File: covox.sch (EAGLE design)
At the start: 26 parts, among them CN1 POWERJACK, IC1 74HCT373N, IC2 74HC164N

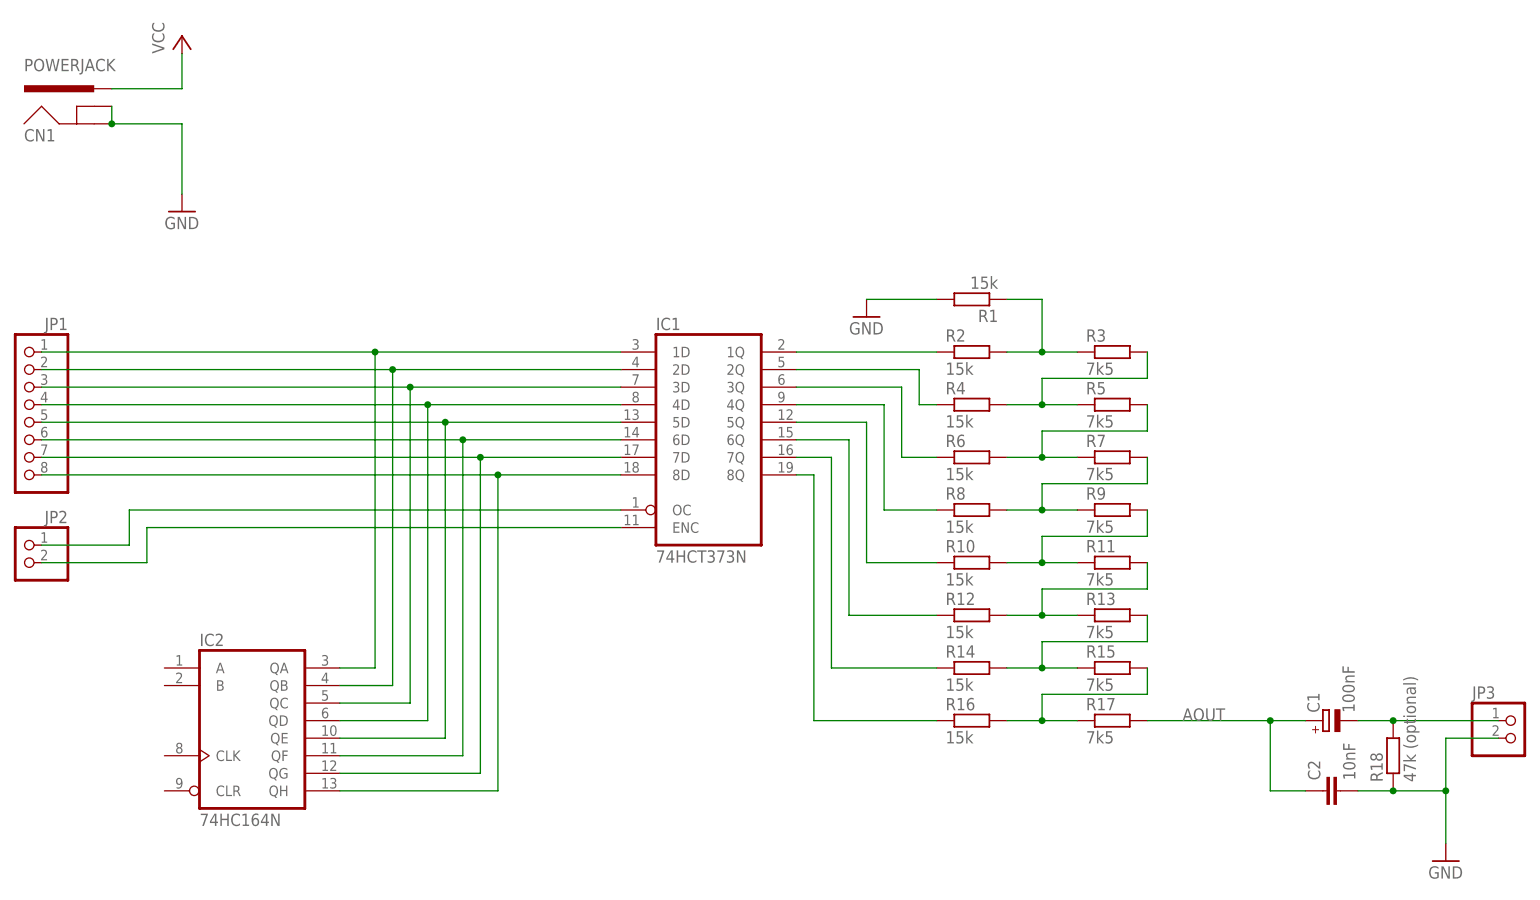
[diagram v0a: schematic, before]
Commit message: Updates...
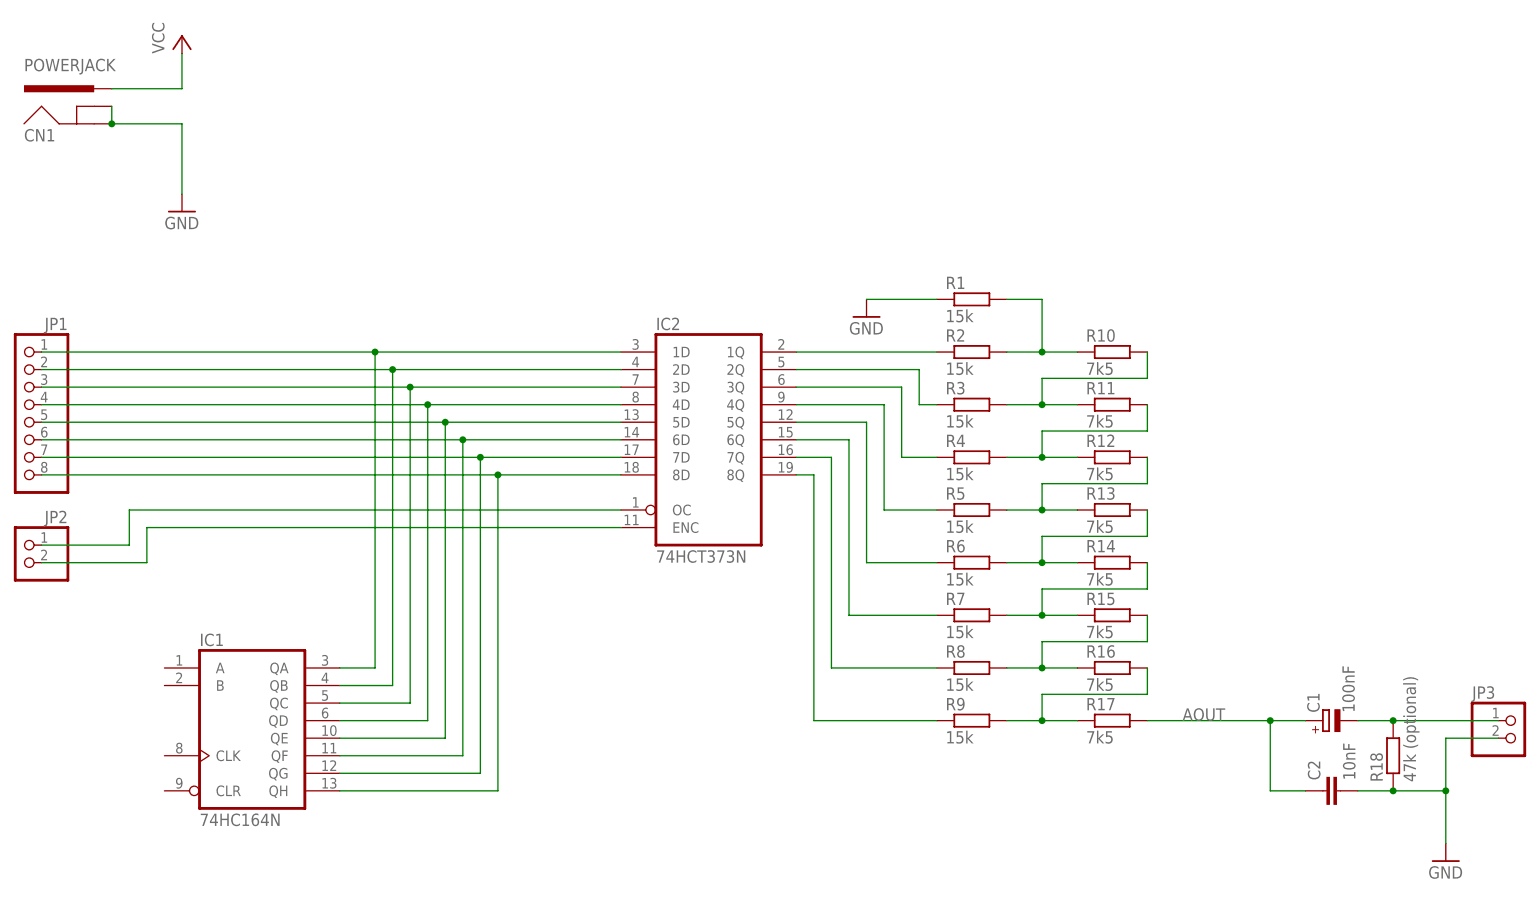
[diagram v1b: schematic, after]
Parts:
- IC1: value 74HCT373N -> 74HC164N; device 74xx-eu:74HCT373N -> 74xx-eu:74HC164N
- IC2: value 74HC164N -> 74HCT373N; device 74xx-eu:74HC164N -> 74xx-eu:74HCT373N
- R10, R12, R14, R16: value 15k -> 7k5
- R3, R5, R7, R9: value 7k5 -> 15k
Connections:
- net GND: now also R1.1; no longer R1.2
- net N$1: now also R1.2, R10.1; no longer R1.1, R3.1
- net N$10: now also IC2A.3Q, R4.1; no longer IC1A.3Q, R6.1
- net N$11: now also IC2A.4Q, R5.1; no longer IC1A.4Q, R8.1
- net N$12: now also IC2A.5Q, R6.1; no longer IC1A.5Q, R10.1
- net N$13: now also IC2A.6Q, R7.1; no longer IC1A.6Q, R12.1
- net N$14: now also IC2A.7Q, R8.1; no longer IC1A.7Q, R14.1
- net N$15: now also IC2A.8Q, R9.1; no longer IC1A.8Q, R16.1
- net N$17: now also R9.2; no longer R15.2
- net N$18: now also IC1A.QA, IC2A.1D; no longer IC1A.1D, IC2A.QA
- net N$19: now also IC1A.QB, IC2A.2D; no longer IC1A.2D, IC2A.QB
- net N$2: now also R10.2, R11.1; no longer R4.2, R5.1
- net N$20: now also IC1A.QC, IC2A.3D; no longer IC1A.3D, IC2A.QC
- net N$21: now also IC1A.QD, IC2A.4D; no longer IC1A.4D, IC2A.QD
- net N$22: now also IC1A.QE, IC2A.5D; no longer IC1A.5D, IC2A.QE
- net N$23: now also IC1A.QF, IC2A.6D; no longer IC1A.6D, IC2A.QF
- net N$24: now also IC1A.QG, IC2A.7D; no longer IC1A.7D, IC2A.QG
- net N$25: now also IC1A.QH, IC2A.8D; no longer IC1A.8D, IC2A.QH
- net N$26: now also IC2A.OC; no longer IC1A.OC
- net N$27: now also IC2A.ENC; no longer IC1A.ENC
- net N$3: now also R11.2, R12.1, R4.2; no longer R5.2, R6.2, R7.1
- net N$4: now also R12.2, R13.1, R5.2; no longer R7.2, R8.2, R9.1
- net N$5: now also R13.2, R14.1, R6.2; no longer R10.2, R11.1, R9.2
- net N$6: now also R14.2, R15.1, R7.2; no longer R11.2, R12.2, R13.1
- net N$7: now also R15.2, R16.1, R8.2; no longer R13.2, R14.2, R15.1
- net N$8: now also IC2A.1Q; no longer IC1A.1Q
- net N$9: now also IC2A.2Q, R3.1; no longer IC1A.2Q, R4.1
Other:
- moved on the sheet: R1, R10, R11, R12, R13, R14, R15, R16, R3, R4, R5, R6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
